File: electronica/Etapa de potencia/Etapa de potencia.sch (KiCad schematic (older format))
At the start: 18 parts, among them J1 Bornera Resorte, J2 Bornera Resorte, J3 Bornera Resorte, J4 Bornera 4 pines, U1 ATmega328-PU, U2 ULN2003, U3 ULN2003, U4 MOC3031M, U5 WeMos_D1_mini, U6 ULN2002A, Y1 Crystal

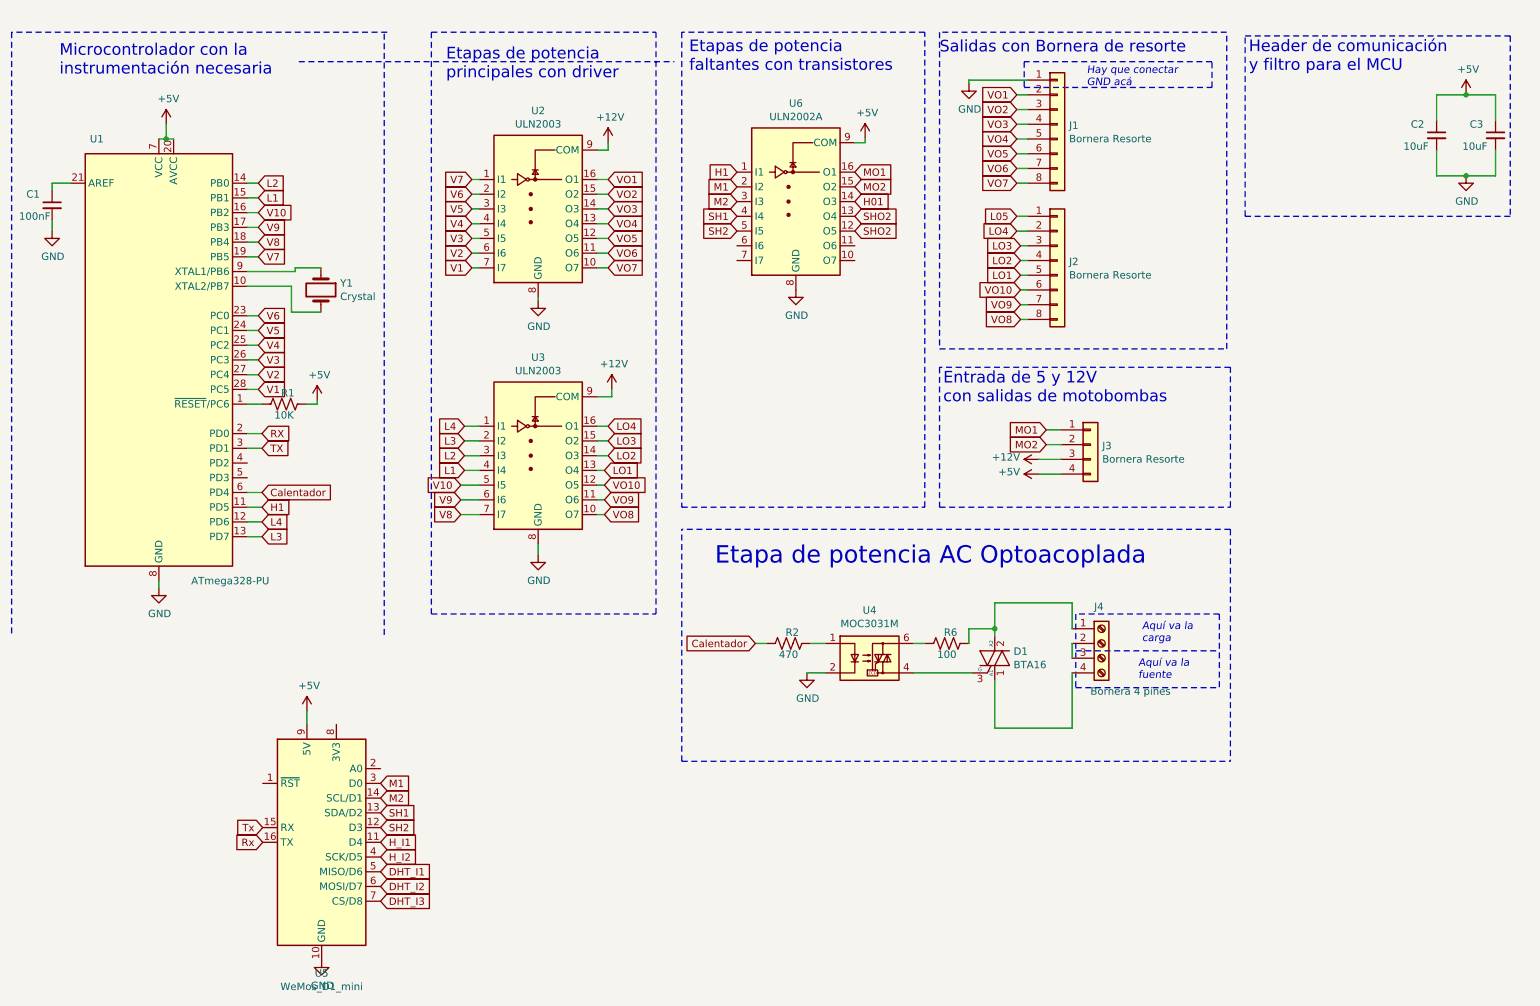
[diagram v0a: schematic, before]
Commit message: ending first pcb
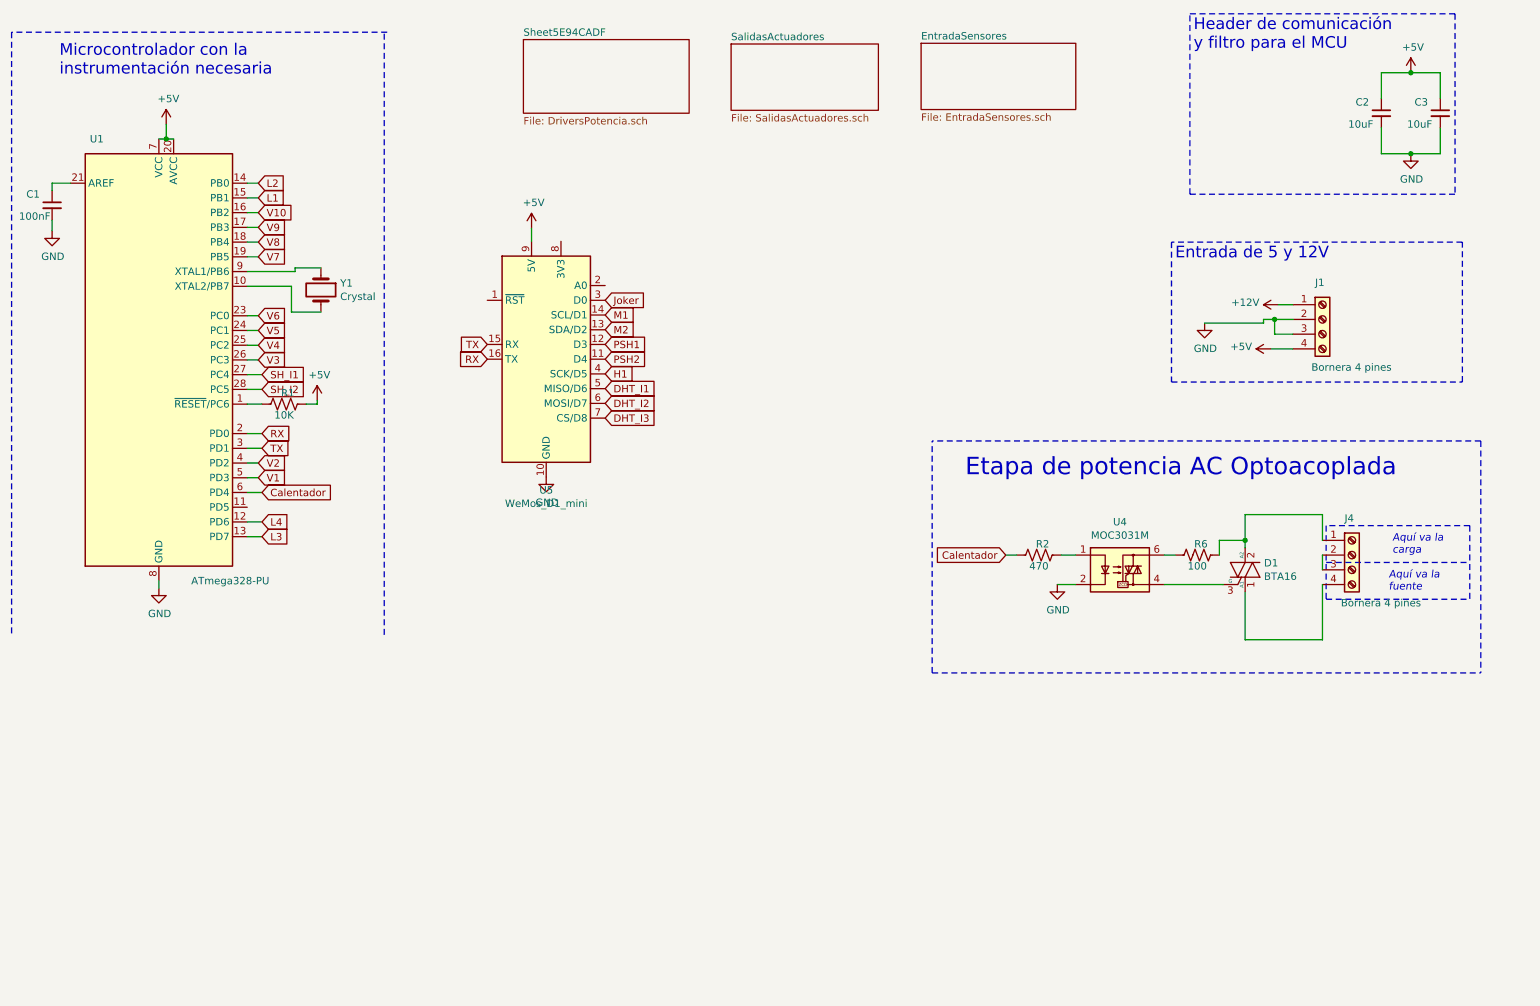
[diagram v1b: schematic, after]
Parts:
- removed J1, J2: Bornera Resorte, potenciaFootprints:BorneraKF141R_8Pins, symbol Connector_Generic:Conn_01x08
- removed J3: Bornera Resorte, potenciaFootprints:BorneraKF141R_4Pins, symbol Connector_Generic:Conn_01x04
- removed U2, U3: ULN2003, Package_DIP:DIP-16_W7.62mm_LongPads, symbol Transistor_Array:ULN2003
- removed U6: ULN2002A, Package_DIP:DIP-16_W7.62mm_LongPads, symbol Transistor_Array:ULN2002A
- added J1: Bornera 4 pines, TerminalBlock:TerminalBlock_Altech_AK300-4_P5.00mm, symbol Connector:Screw_Terminal_01x04
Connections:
- net H_I2 is gone; now on net H1: U5.4 (SCK/D5)
- net Rx is gone; now on net RX: U5.16 (TX)
- net SH1 is gone; now on net M2: U5.13 (SDA/D2)
- net Tx is gone; now on net TX: U5.15 (RX)
- net +12V: now also J1.1 (Pin_1)
- net +5V: now also J1.4 (Pin_4)
- net GND: now also J1.2 (Pin_2), J1.3 (Pin_3)
- net H1: no longer U1.11 (PD5)
- net M1: now also U5.14 (SCL/D1); no longer U5.3 (D0)
- net M2: no longer U5.14 (SCL/D1)
- net V1: now also U1.5 (PD3); no longer U1.28 (PC5)
- net V2: now also U1.4 (PD2); no longer U1.27 (PC4)
- net H_I1 renamed PSH2
- net SH2 renamed PSH1
- new net Joker: U5.3 (D0)
- new net SH_I1: U1.27 (PC4)
- new net SH_I2: U1.28 (PC5)
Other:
- note added: "Entrada de 5 y 12V\n\n"
- note removed: "Entrada de 5 y 12V\ncon salidas de motobombas\n"
- note removed: "Etapas de potencia \nfaltantes con transistores"
- note removed: "Etapas de potencia \nprincipales con driver"
- note removed: "Hay que conectar \nGND acá"
- note removed: "Salidas con Bornera de resorte"
- moved on the sheet: C2, C3, D1, J4, R2, R6, U4, U5
